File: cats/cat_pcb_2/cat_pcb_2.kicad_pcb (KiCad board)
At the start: 2 copper layers, 43.5 x 64 mm, 6 parts, among them SW1 SMT_SPDT

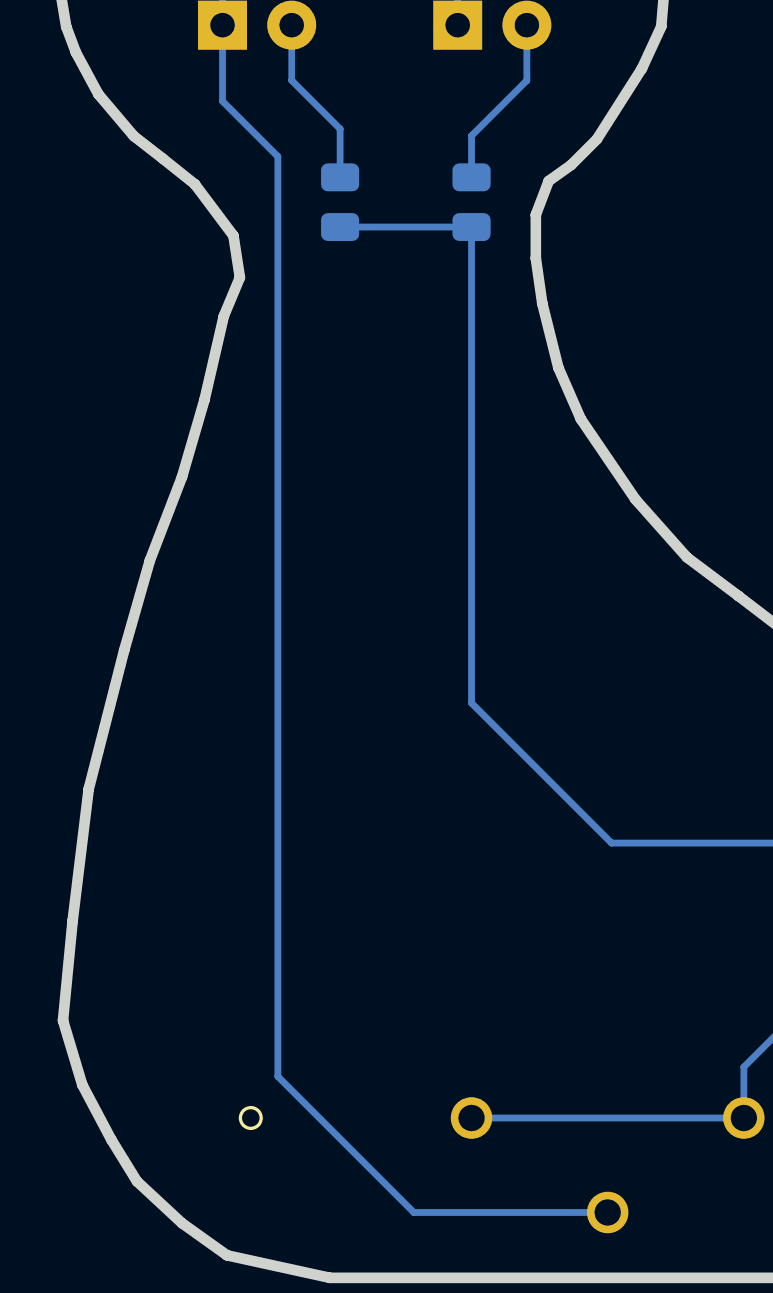
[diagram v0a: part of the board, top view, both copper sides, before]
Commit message: Bunch of changes
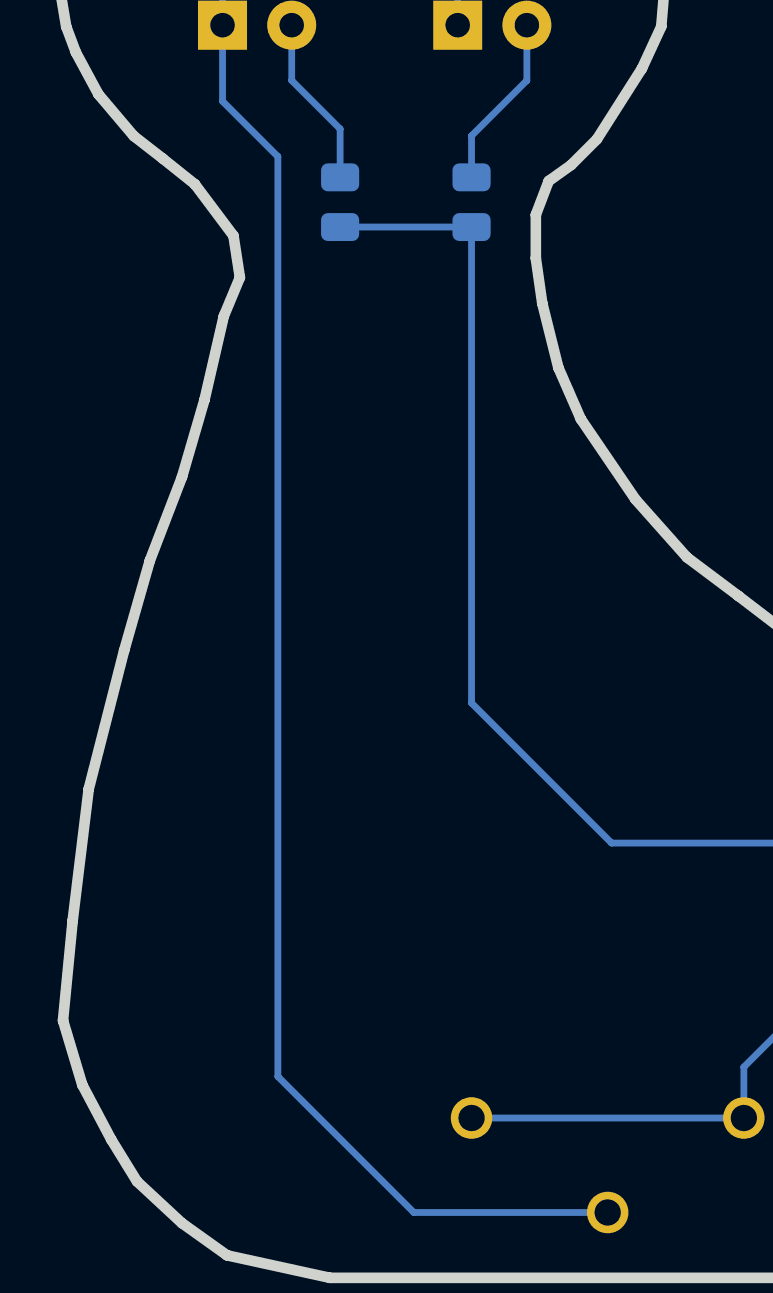
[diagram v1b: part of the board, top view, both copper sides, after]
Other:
- board text added: "+ POSITIVE +"
